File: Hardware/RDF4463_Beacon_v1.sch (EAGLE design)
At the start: 12 parts, among them M1 DORJI_DRF4463F, U1 PIC18F24K22

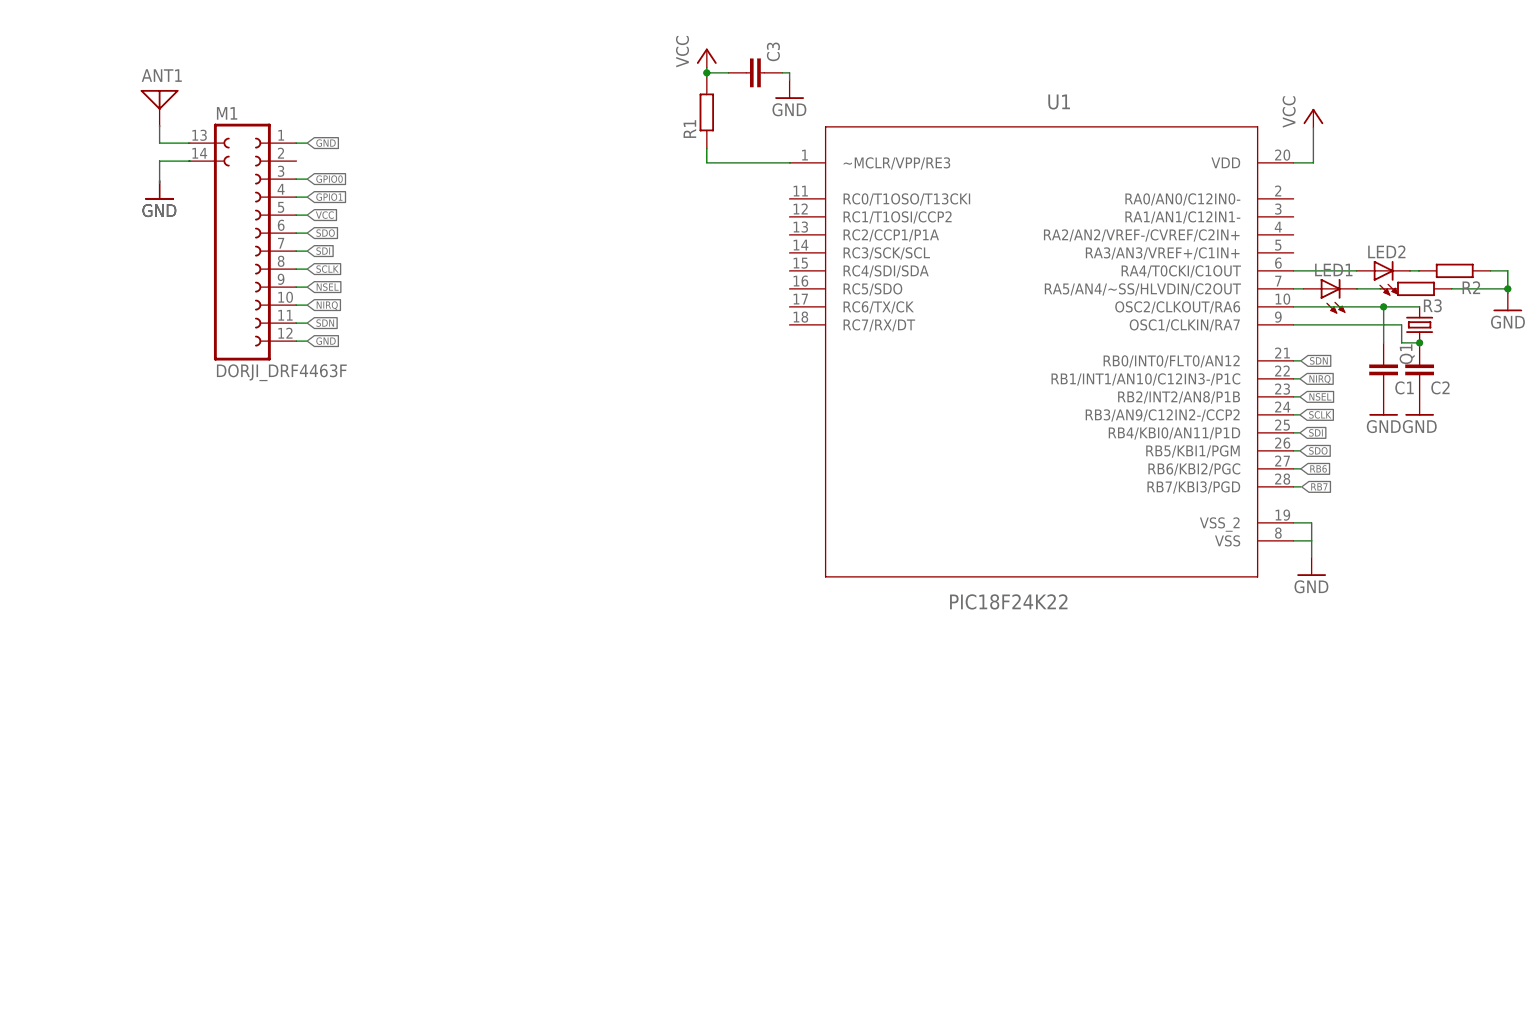
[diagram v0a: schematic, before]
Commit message: Guncelleme
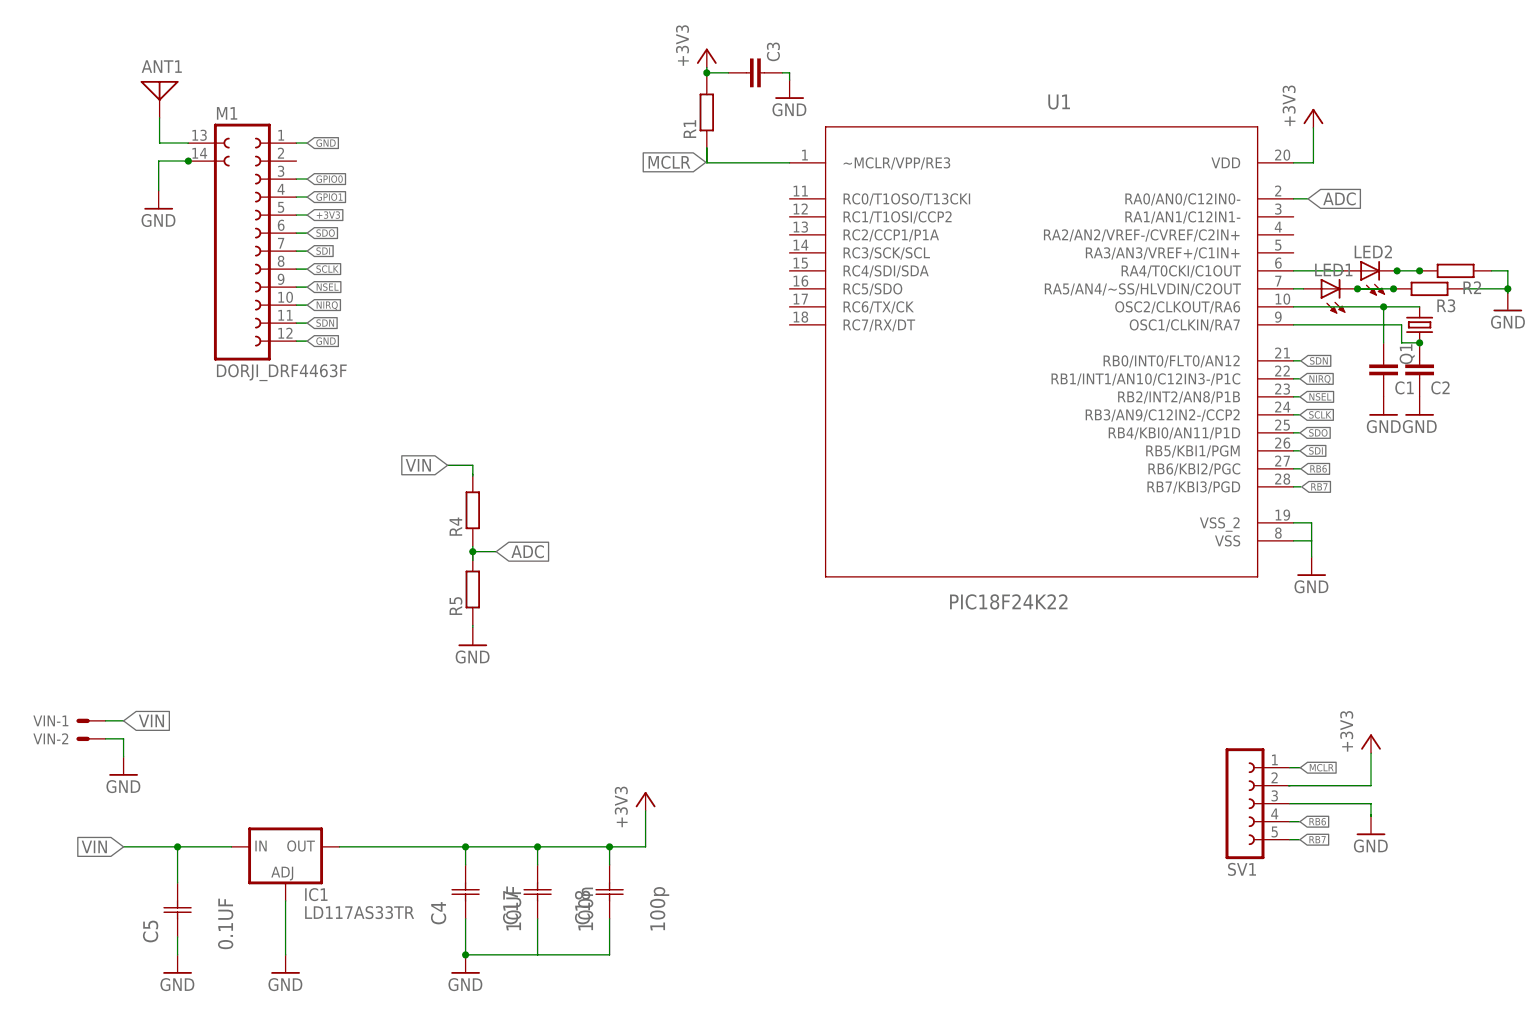
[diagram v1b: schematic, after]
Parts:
- added C17: 100n, AVX_By_element14_Batch_1:0805YD106MAT2A
- added C18: 100p, AVX_By_element14_Batch_1:0805YD106MAT2A
- added C4: 10UF, AVX_By_element14_Batch_1:0805YD106MAT2A
- added C5: 0.1UF, AVX_By_element14_Batch_1:0805ZC104MAT2A
- added IC1: LD117AS33TR, v-reg:LD117AS33TR
- added R4, R5: (no value), rcl:R-EU_R0805
- added SV1: (no value), con-lsta:FE05-1
- added VIN: (no value), con-molex:KK-156-2
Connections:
- new net +3V3: C17.C2, C18.C2, C4.C2, IC1.OUT, M1.5
- new net ADC: R4.1, R5.2, U1.RA0/AN0/C12IN0-
- new net MCLR: SV1.1, U1.~MCLR/VPP/RE3
- new net N$2: ANT1.1, M1.13
- new net N$8: LED2.C, R2.2
- new net RB6: SV1.4
- new net VIN: C5.C2, IC1.IN, R4.2, VIN-1.S
- net GND: now also C17.C1, C18.C1, C4.C1, C5.C1, IC1.ADJ, M1.14, R5.1, SV1.3, VIN-2.S
- net N$9: now also LED1.C
- net RB7: now also SV1.5
- net SDI: now also U1.RB5/KBI1/PGM; no longer U1.RB4/KBI0/AN11/P1D
- net SDO: now also U1.RB4/KBI0/AN11/P1D; no longer U1.RB5/KBI1/PGM
- net VCC: now also SV1.2; no longer M1.5
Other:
- moved on the sheet: ANT1, LED2, R3
